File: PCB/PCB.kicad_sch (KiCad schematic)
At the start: 6 parts, among them P1 USB_C_Plug_USB2.0, Q1 BC549C

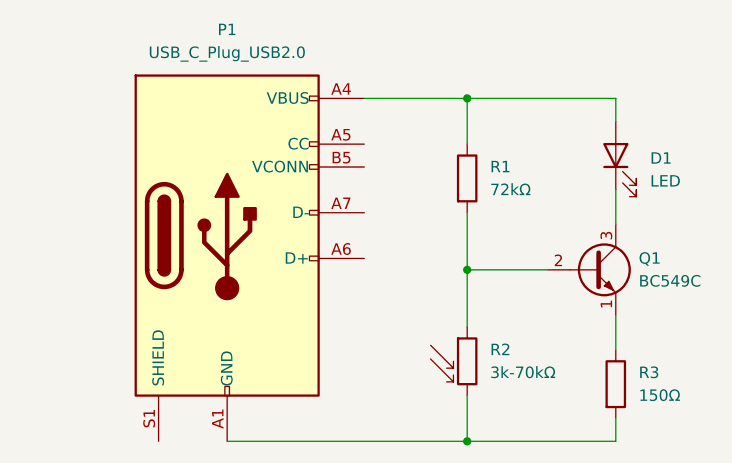
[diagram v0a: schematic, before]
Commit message: Reroute PCB
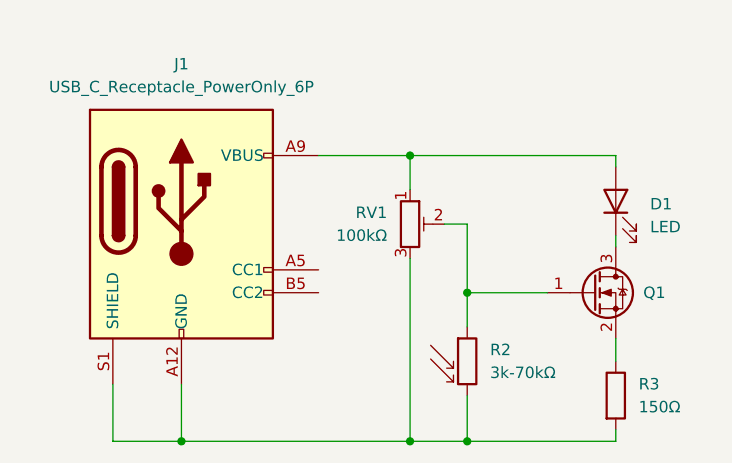
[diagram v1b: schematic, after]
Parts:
- removed P1: USB_C_Plug_USB2.0, Connector_USB:USB_C_Receptacle_GCT_USB4105-xx-A_16P_TopMnt_Horizontal, symbol Connector:USB_C_Plug_USB2.0
- removed Q1: BC549C, Package_TO_SOT_THT:TO-92_Inline_Wide, symbol Transistor_BJT:BC107
- removed R1: 72kΩ, Resistor_THT:R_Axial_DIN0207_L6.3mm_D2.5mm_P15.24mm_Horizontal, symbol Device:R
- added J1: USB_C_Receptacle_PowerOnly_6P, Connector_USB:USB_C_Receptacle_GCT_USB4125-xx-x-0190_6P_TopMnt_Horizontal, symbol Connector:USB_C_Receptacle_PowerOnly_6P
- added Q1: ~, Package_TO_SOT_SMD:SOT-23, symbol Transistor_FET:T2N7002AK
- added RV1: 100kΩ, Potentiometer_SMD:Potentiometer_Bourns_TC33X_Vertical, symbol Device:R_Potentiometer_Trim
- R2: footprint OptoDevice:R_LDR_10x8.5mm_P7.6mm_Vertical -> OptoDevice:R_LDR_5.1x4.3mm_P3.4mm_Vertical
- R3: footprint Resistor_THT:R_Axial_DIN0207_L6.3mm_D2.5mm_P15.24mm_Horizontal -> Resistor_SMD:R_0402_1005Metric
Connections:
- net at R2.1: now also Q1.1 (G), RV1.2
- net at R2.2, R3.2: now also J1.A12 (GND), J1.B12 (GND), J1.S1 (SHIELD), RV1.3
- net at R3.1: now also Q1.2 (S)
- net at D1.1 (K): now also Q1.3 (D)
- net at D1.2 (A): now also J1.A9 (VBUS), J1.B9 (VBUS), RV1.1
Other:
- moved on the sheet: D1, R3
